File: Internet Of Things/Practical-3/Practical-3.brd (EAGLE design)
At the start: 82.4 x 106.9 mm, 4 parts, among them U1 ARDUINO-UNO-R3-SHIELD, U2 TMP36GT9Z_TO92

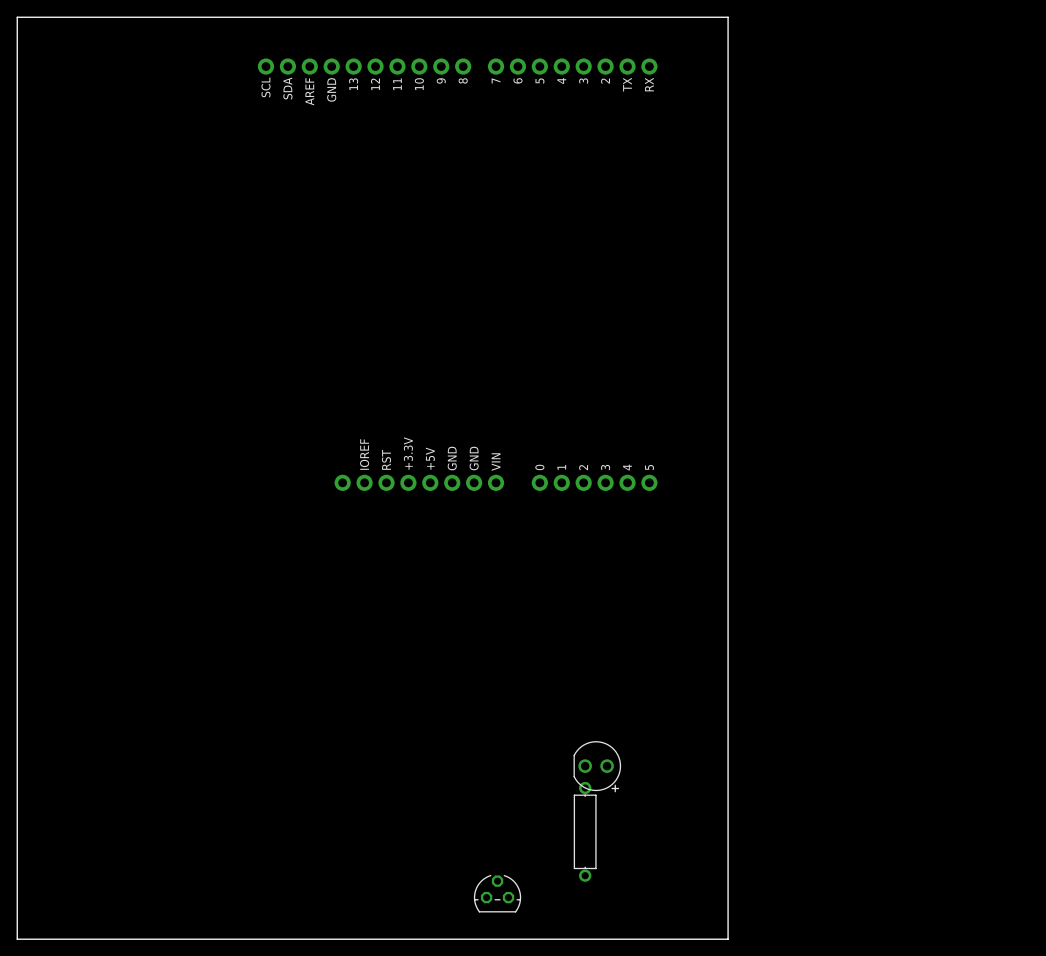
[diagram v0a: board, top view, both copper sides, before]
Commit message: Modified the practical-3 files
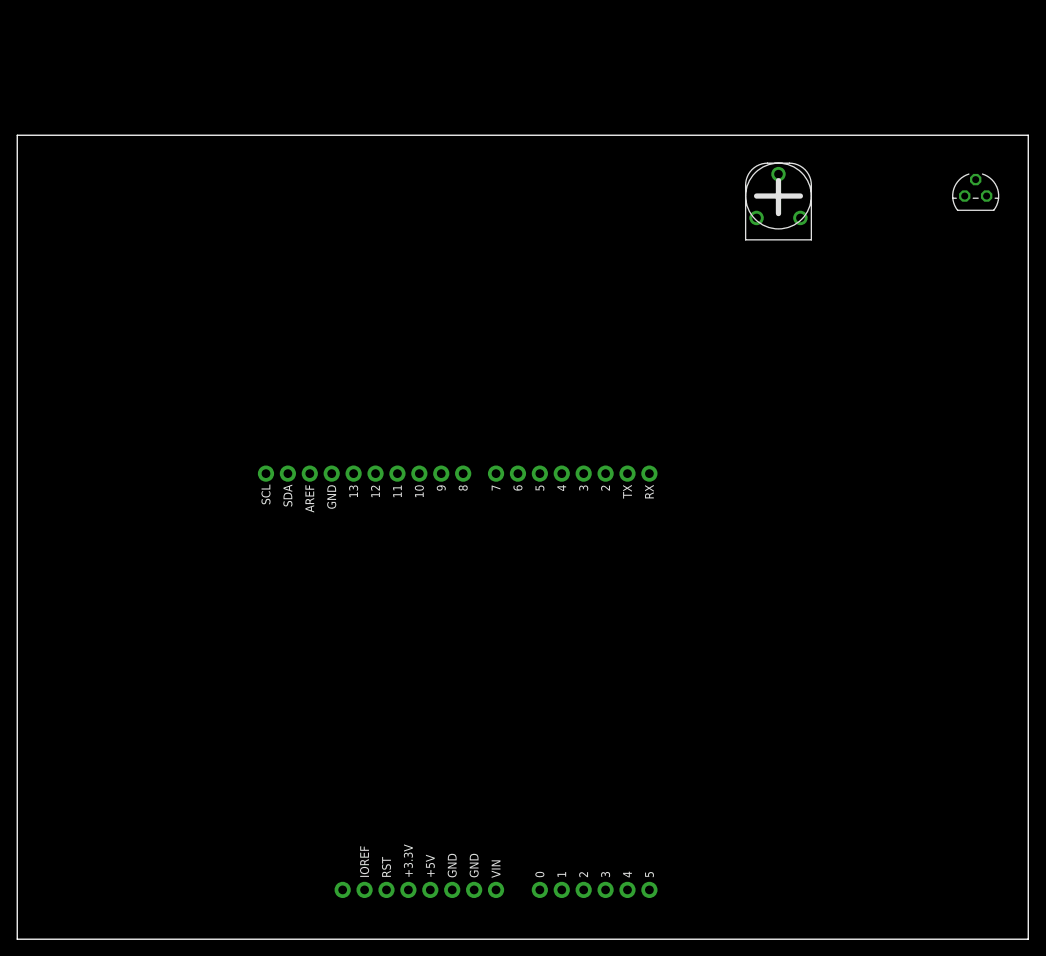
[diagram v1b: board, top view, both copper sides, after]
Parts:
- removed D1: RED, Tinkercad:LEDRD254W60D565H860B
- removed R1: 1k, Tinkercad:RESAD1016W63L850D250B
- added RPOT1: 250k, Tinkercad:HA-06-SM065
- U1: value ARDUINO-UNO-R3-SHIELD -> TMP36GT9Z_TO92; device Tinkercad:ARDUINO-UNO-R3-SHIELD -> Tinkercad:TO92
- U2: value TMP36GT9Z_TO92 -> ARDUINO-UNO-R3-SHIELD; device Tinkercad:TO92 -> Tinkercad:ARDUINO-UNO-R3-SHIELD
- moved U1 63.9 mm to (111.1, 86.2), turned to 0 degrees
- moved U2 26.2 mm to (47.9, 29.8), turned to 270 degrees
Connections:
- removed net D1_C: D1.2, R1.2
- removed net U1_5V: U1.5V, U2.3
- removed net U1_A0: U1.A0, U2.2
- removed net U1_D13: D1.1, U1.D13
- removed net U1_GND: R1.1, U1.GND@0, U1.GND@1, U1.GND@2, U2.1
- new net U2_5V: RPOT1.3, U1.1, U2.5V
- new net U2_A0: RPOT1.2, U2.A0
- new net U2_A1: U1.2, U2.A1
- new net U2_GND: RPOT1.1, U1.3, U2.GND@0, U2.GND@1, U2.GND@2
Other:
- board size 82.4 x 106.9 mm -> 117.2 x 93.2 mm
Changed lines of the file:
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@@
 <board>
 <plain>
-<wire x1="0" y1="0" x2="82.40360000000001" y2="0" width="0" layer="20"/>
-<wire x1="82.40360000000001" y1="0" x2="82.40360000000001" y2="106.8805918719356" width="0" layer="20"/>
-<wire x1="82.40360000000001" y1="106.8805918719356" x2="0" y2="106.8805918719356" width="0" layer="20"/>
-<wire x1="0" y1="106.8805918719356" x2="0" y2="0" width="0" layer="20"/>
+<wire x1="0" y1="0" x2="117.20532786639048" y2="0" width="0" layer="20"/>
+<wire x1="117.20532786639048" y1="0" x2="117.20532786639048" y2="93.20279879697215" width="0" layer="20"/>
+<wire x1="117.20532786639048" y1="93.20279879697215" x2="0" y2="93.20279879697215" width="0" layer="20"/>
+<wire x1="0" y1="93.20279879697215" x2="0" y2="0" width="0" layer="20"/>
 </plain>
 <attributes/>
@@
 </autorouter>
 <elements>
-<element name="U2" library="Tinkercad" package="TO92" package3d_urn="urn:adsk.eagle:package:16378726/12" value="TMP36GT9Z_TO92" x="55.6784" y="4.826" smashed="yes"/>
-<element name="U1" library="Tinkercad" package="ARDUINO-UNO-R3-SHIELD" package3d_urn="urn:adsk.eagle:package:32092383/4" value="ARDUINO-UNO-R3-SHIELD" x="47.885" y="77.0356" rot="R270" smashed="yes"/>
-<element name="R1" library="Tinkercad" package="RESAD1016W63L850D250B" package3d_urn="urn:adsk.eagle:package:31513020/2" value="1k" x="65.8384" y="12.446" rot="R90" smashed="yes"/>
-<element name="D1" library="Tinkercad" package="LEDRD254W60D565H860B" package3d_urn="urn:adsk.eagle:package:16378508/2" value="RED" x="67.1084" y="20.066" rot="R180" smashed="yes">
-<attribute name="CATEGORY" value="Opto-Electronic" x="67.1084" y="20.066" size="1.778" layer="27" display="off"/>
-<attribute name="COLOR" value="" x="67.1084" y="20.066" size="1.778" layer="27" display="off"/>
-<attribute name="DESCRIPTION" value="" x="67.1084" y="20.066" size="1.778" layer="27" display="off"/>
-<attribute name="MANUFACTURER" value="" x="67.1084" y="20.066" size="1.778" layer="27" display="off"/>
-<attribute name="MPN" value="" x="67.1084" y="20.066" size="1.778" layer="27" display="off"/>
-<attribute name="OPERATING_TEMP" value="" x="67.1084" y="20.066" size="1.778" layer="27" display="off"/>
-<attribute name="PART_STATUS" value="" x="67.1084" y="20.066" size="1.778" layer="27" display="off"/>
-<attribute name="ROHS_COMPLIANT" value="" x="67.1084" y="20.066" size="1.778" layer="27" display="off"/>
-<attribute name="SERIES" value="" x="67.1084" y="20.066" size="1.778" layer="27" display="off"/>
-<attribute name="SUB-CATEGORY" value="LED" x="67.1084" y="20.066" size="1.778" layer="27" display="off"/>
-<attribute name="THERMALLOSS" value="" x="67.1084" y="20.066" size="1.778" layer="27" display="off"/>
-<attribute name="TYPE" value="" x="67.1084" y="20.066" size="1.778" layer="27" display="off"/>
-<attribute name="VALUE" value="LED_RED" x="67.1084" y="20.066" size="1.778" layer="27" display="off"/>
-</element>
+<element name="U1" library="Tinkercad" package="TO92" package3d_urn="urn:adsk.eagle:package:16378726/12" value="TMP36GT9Z_TO92" x="111.1093" y="86.1543" smashed="yes"/>
+<element name="U2" library="Tinkercad" package="ARDUINO-UNO-R3-SHIELD" package3d_urn="urn:adsk.eagle:package:32092383/4" value="ARDUINO-UNO-R3-SHIELD" x="47.885" y="29.845" rot="R270" smashed="yes"/>
+<element name="RPOT1" library="Tinkercad" package="HA-06-SM065" package3d_urn="urn:adsk.eagle:package:31496083/2" value="250k" x="88.2493" y="86.1543" smashed="yes"/>
 </elements>
 <signals>
-<signal name="U1_GND">
-<contactref element="R1" pad="1"/>
-<contactref element="U2" pad="1"/>
-<contactref element="U1" pad="GND@0"/>
-<contactref element="U1" pad="GND@1"/>
-<contactref element="U1" pad="GND@2"/>
-<wire x1="50.425" y1="52.9056" x2="52.965" y2="52.9056" width="0" layer="19" extent="1-1"/>
-<wire x1="65.8384" y1="7.366" x2="52.965" y2="52.9056" width="0" layer="19" extent="1-1"/>
-<wire x1="65.8384" y1="7.366" x2="54.4084" y2="4.826" width="0" layer="19" extent="1-1"/>
-<wire x1="50.425" y1="52.9056" x2="36.455" y2="101.1656" width="0" layer="19" extent="1-1"/>
-</signal>
-<signal name="U1_A0">
-<contactref element="U2" pad="2"/>
-<contactref element="U1" pad="A0"/>
-<wire x1="55.6784" y1="6.731" x2="60.585" y2="52.9056" width="0" layer="19" extent="1-1"/>
-</signal>
-<signal name="U1_5V">
-<contactref element="U2" pad="3"/>
-<contactref element="U1" pad="5V"/>
-<wire x1="56.9484" y1="4.826" x2="47.885" y2="52.9056" width="0" layer="19" extent="1-1"/>
-</signal>
-<signal name="U1_D13">
-<contactref element="U1" pad="D13"/>
-<contactref element="D1" pad="1"/>
-<wire x1="38.995" y1="101.1656" x2="68.3784" y2="20.066" width="0" layer="19" extent="1-1"/>
-</signal>
-<signal name="D1_C">
-<contactref element="D1" pad="2"/>
-<contactref element="R1" pad="2"/>
-<wire x1="65.8384" y1="20.066" x2="65.8384" y2="17.526" width="0" layer="19" extent="1-1"/>
+<signal name="U2_5V">
+<contactref element="U1" pad="1"/>
+<contactref element="RPOT1" pad="3"/>
+<contactref element="U2" pad="5V"/>
+<wire x1="109.8393" y1="86.1543" x2="90.7893" y2="83.6143" width="0" layer="19" extent="1-1"/>
+<wire x1="90.7893" y1="83.6143" x2="47.885" y2="5.715" width="0" layer="19" extent="1-1"/>
+</signal>
+<signal name="U2_A1">
+<contactref element="U1" pad="2"/>
+<contactref element="U2" pad="A1"/>
+<wire x1="111.1093" y1="88.0593" x2="63.125" y2="5.715" width="0" layer="19" extent="1-1"/>
+</signal>
+<signal name="U2_GND">
+<contactref element="U1" pad="3"/>
+<contactref element="RPOT1" pad="1"/>
+<contactref element="U2" pad="GND@0"/>
+<contactref element="U2" pad="GND@1"/>
+<contactref element="U2" pad="GND@2"/>
+<wire x1="50.425" y1="5.715" x2="52.965" y2="5.715" width="0" layer="19" extent="1-1"/>
+<wire x1="50.425" y1="5.715" x2="36.455" y2="53.975" width="0" layer="19" extent="1-1"/>
+<wire x1="85.7093" y1="83.6143" x2="36.455" y2="53.975" width="0" layer="19" extent="1-1"/>
+<wire x1="112.3793" y1="86.1543" x2="85.7093" y2="83.6143" width="0" layer="19" extent="1-1"/>
+</signal>
+<signal name="U2_A0">
+<contactref element="RPOT1" pad="2"/>
+<contactref element="U2" pad="A0"/>
+<wire x1="88.2493" y1="88.6943" x2="60.585" y2="5.715" width="0" layer="19" extent="1-1"/>
 </signal>
 </signals>
